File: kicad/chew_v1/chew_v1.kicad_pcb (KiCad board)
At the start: 2 copper layers, 160.3 x 91.9 mm, 44 parts, among them J2 AudioJack4dpb, SW1 SW_Push, SW10 SW_Push, SW11 SW_Push, SW12 SW_Push, SW13 SW_Push, SW14 SW_Push, SW15 SW_Push, SW16 SW_Push, SW17 SW_Push, SW2 SW_Push, SW3 SW_Push, SW4 SW_Push, SW5 SW_Push, SW6 SW_Push, SW7 SW_Push, SW8 SW_Push, SW9 SW_Push

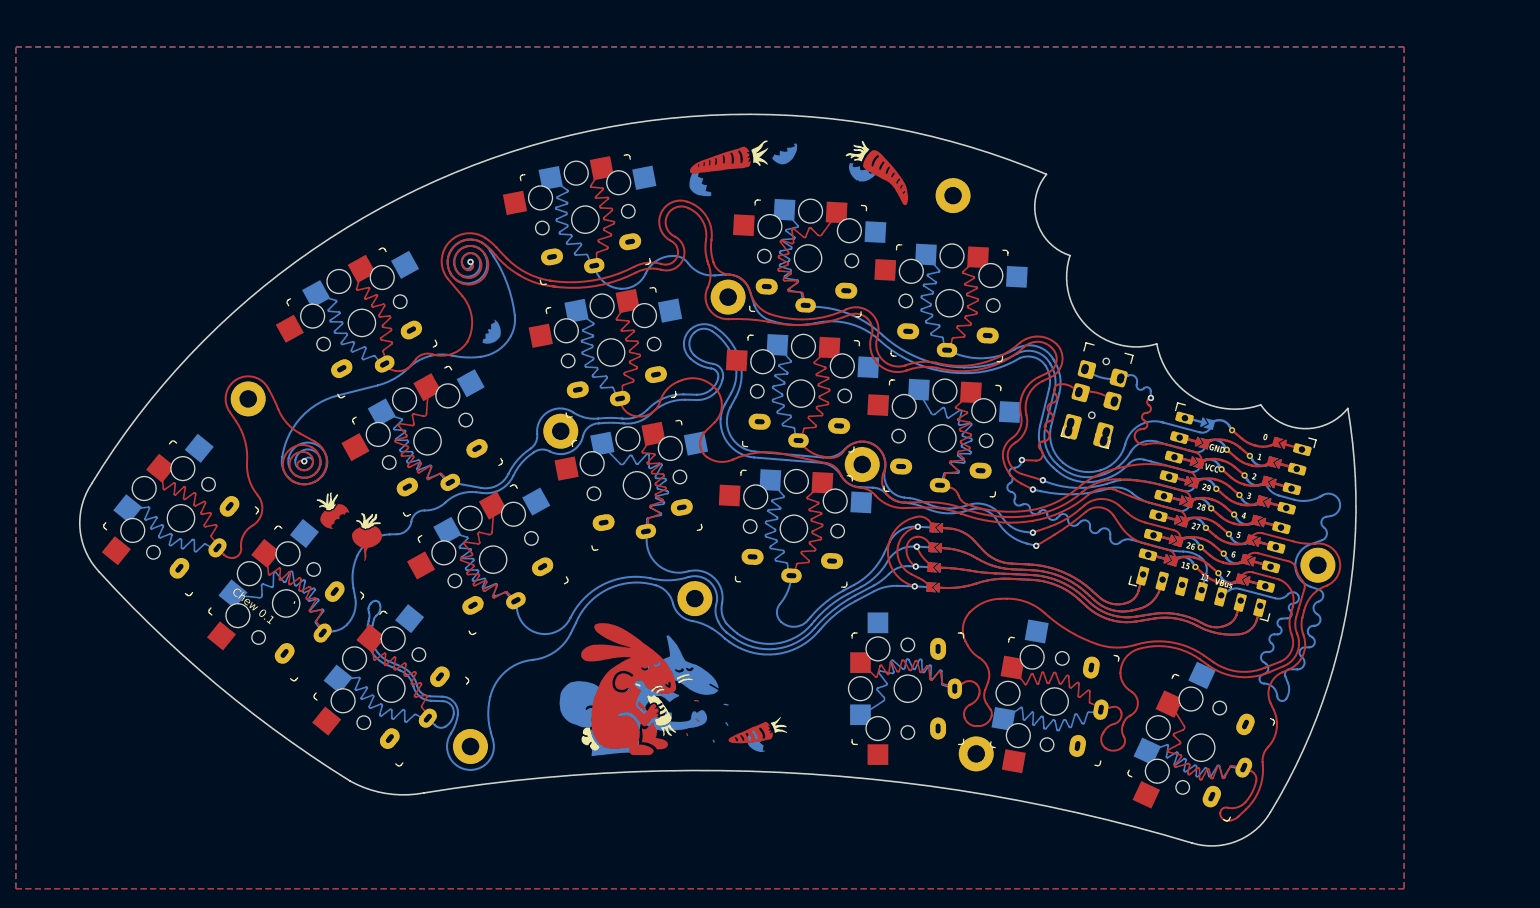
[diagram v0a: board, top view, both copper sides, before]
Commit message: Create libs
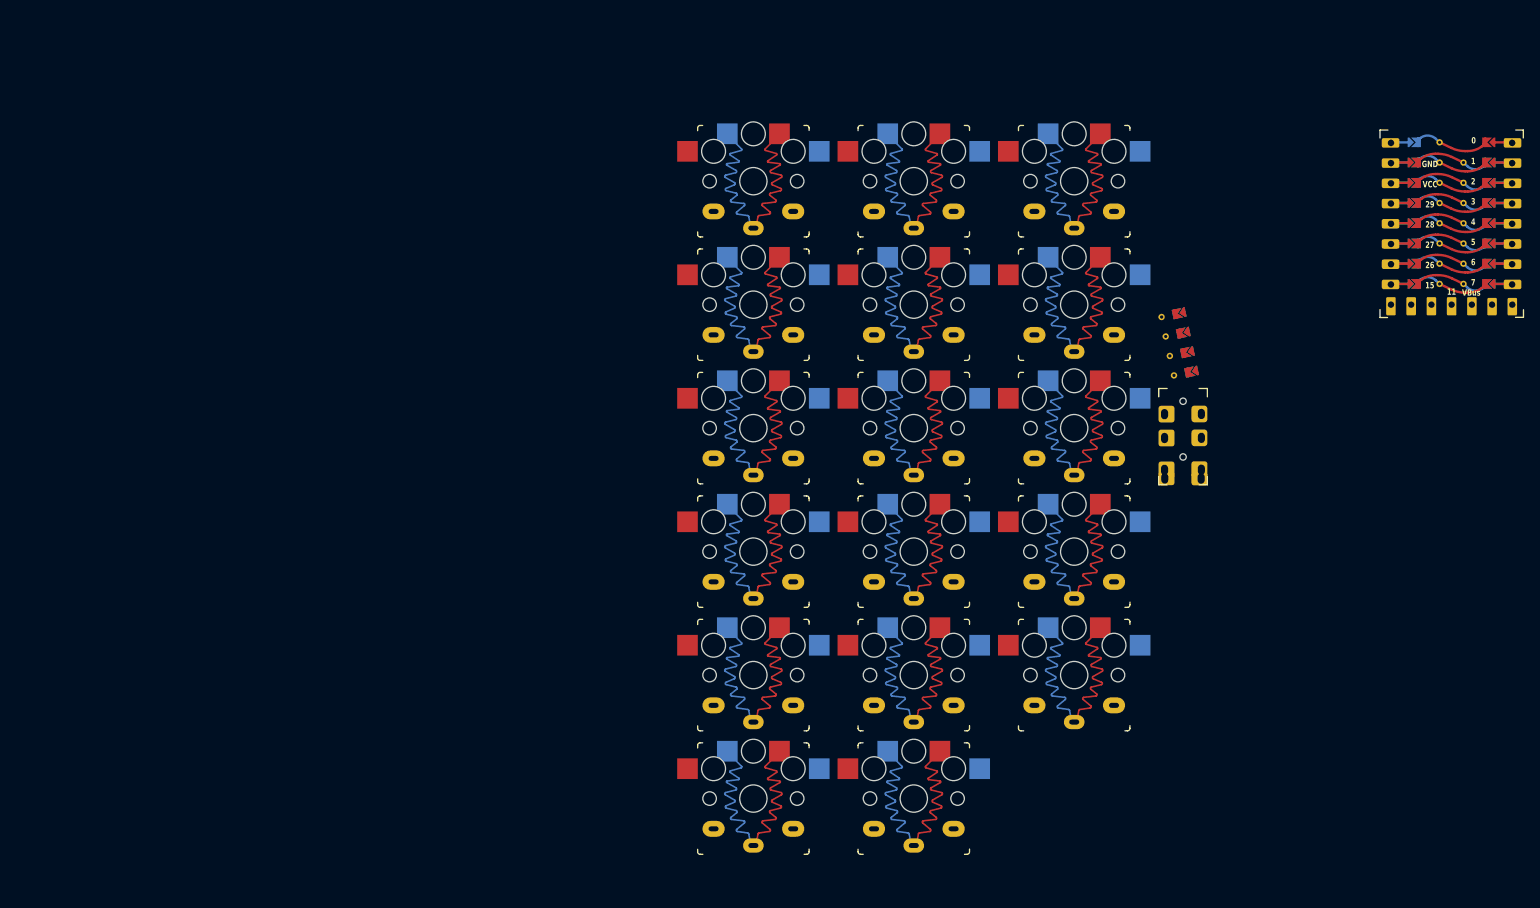
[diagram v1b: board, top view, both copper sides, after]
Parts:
- removed ? (x4): , clipboard:420c2a85-5b5b-48ff-b81a-8100f601aced
- removed ? (x5): , 
- removed G*** (x15): LOGO, LOGO
- removed J2: AudioJack4dpb, Kailh:TRRS-PJ-DPB2
- removed REF**: Tenting Puck, kbd:Tenting_Puck2
- removed RZ1: RP2040-Zero, BumWings_Library:RP2040-Zero
- removed SW1, SW10, SW11, SW12, SW13, SW14, SW15, SW16, SW17, SW2, SW3, SW4, SW5, SW6, SW7, SW8, SW9: SW_Push, * duckyb-collection:SW_PG1350_rev_DPB
- added S1: Keyswitch, chew_is_so:Choc_V1_chew_reversible_1, F.Cu at (113.7, 60.8)
- added S10: Keyswitch, chew_is_so:Choc_V1_chew_reversible_1, F.Cu at (133.9, 107.3)
- added S11: Keyswitch, chew_is_so:Choc_V1_chew_reversible_1, F.Cu at (133.9, 122.8)
- added S12: Keyswitch, chew_is_so:Choc_V1_chew_reversible_1, F.Cu at (133.9, 138.3)
- added S13: Keyswitch, chew_is_so:Choc_V1_chew_reversible_1, F.Cu at (154.0, 60.8)
- added S14: Keyswitch, chew_is_so:Choc_V1_chew_reversible_1, F.Cu at (154.0, 76.3)
- added S15: Keyswitch, chew_is_so:Choc_V1_chew_reversible_1, F.Cu at (154.0, 91.8)
- added S16: Keyswitch, chew_is_so:Choc_V1_chew_reversible_1, F.Cu at (154.0, 107.3)
- added S17: Keyswitch, chew_is_so:Choc_V1_chew_reversible_1, F.Cu at (154.0, 122.8)
- added S2: Keyswitch, chew_is_so:Choc_V1_chew_reversible_1, F.Cu at (113.7, 76.3)
- added S3: Keyswitch, chew_is_so:Choc_V1_chew_reversible_1, F.Cu at (113.7, 91.8)
- added S4: Keyswitch, chew_is_so:Choc_V1_chew_reversible_1, F.Cu at (113.7, 107.3)
- added S5: Keyswitch, chew_is_so:Choc_V1_chew_reversible_1, F.Cu at (113.7, 122.8)
- added S6: Keyswitch, chew_is_so:Choc_V1_chew_reversible_1, F.Cu at (113.7, 138.3)
- added S7: Keyswitch, chew_is_so:Choc_V1_chew_reversible_1, F.Cu at (133.9, 60.8)
- added S8: Keyswitch, chew_is_so:Choc_V1_chew_reversible_1, F.Cu at (133.9, 76.3)
- added S9: Keyswitch, chew_is_so:Choc_V1_chew_reversible_1, F.Cu at (133.9, 91.8)
- added U1: RP2040_Zero, chew_is_so:RP2040_Zero_chew_reversible, F.Cu at (201.4, 66.1)
- added U2: TRRS, chew_is_so:TRRS_chew_reversible, F.Cu at (167.7, 86.8)
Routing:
- net Switch5: track 350.1 -> 0.00 mm, vias 3 -> 0
- net (no net): track 298.2 -> 0.00 mm
- net Switch4: track 169.7 -> 0.00 mm, vias 1 -> 0
- net Switch10: track 157.6 -> 0.00 mm, vias 1 -> 0
- net Switch14: track 144.3 -> 0.00 mm, vias 1 -> 0
- net Switch9: track 133.9 -> 0.00 mm, vias 1 -> 0
- net vcc: track 103.5 -> 0.00 mm, vias 1 -> 0
- net Switch3: track 99.3 -> 0.00 mm
- net Switch8: track 90.2 -> 0.00 mm
- net Switch17: track 86.0 -> 0.00 mm
- net Switch13: track 72.1 -> 0.00 mm, vias 1 -> 0
- net Switch2: track 67.7 -> 0.00 mm
- net Switch16: track 65.5 -> 0.00 mm
- net Switch15: track 61.7 -> 0.00 mm
- net Switch18: track 61.5 -> 0.00 mm, vias 1 -> 0
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- removed copper zone on B.Cu, net gnd
- removed copper zone on F.Cu, net gnd
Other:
- board outline removed
- board text removed: "Chew 0.1"

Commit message: Replace footprints
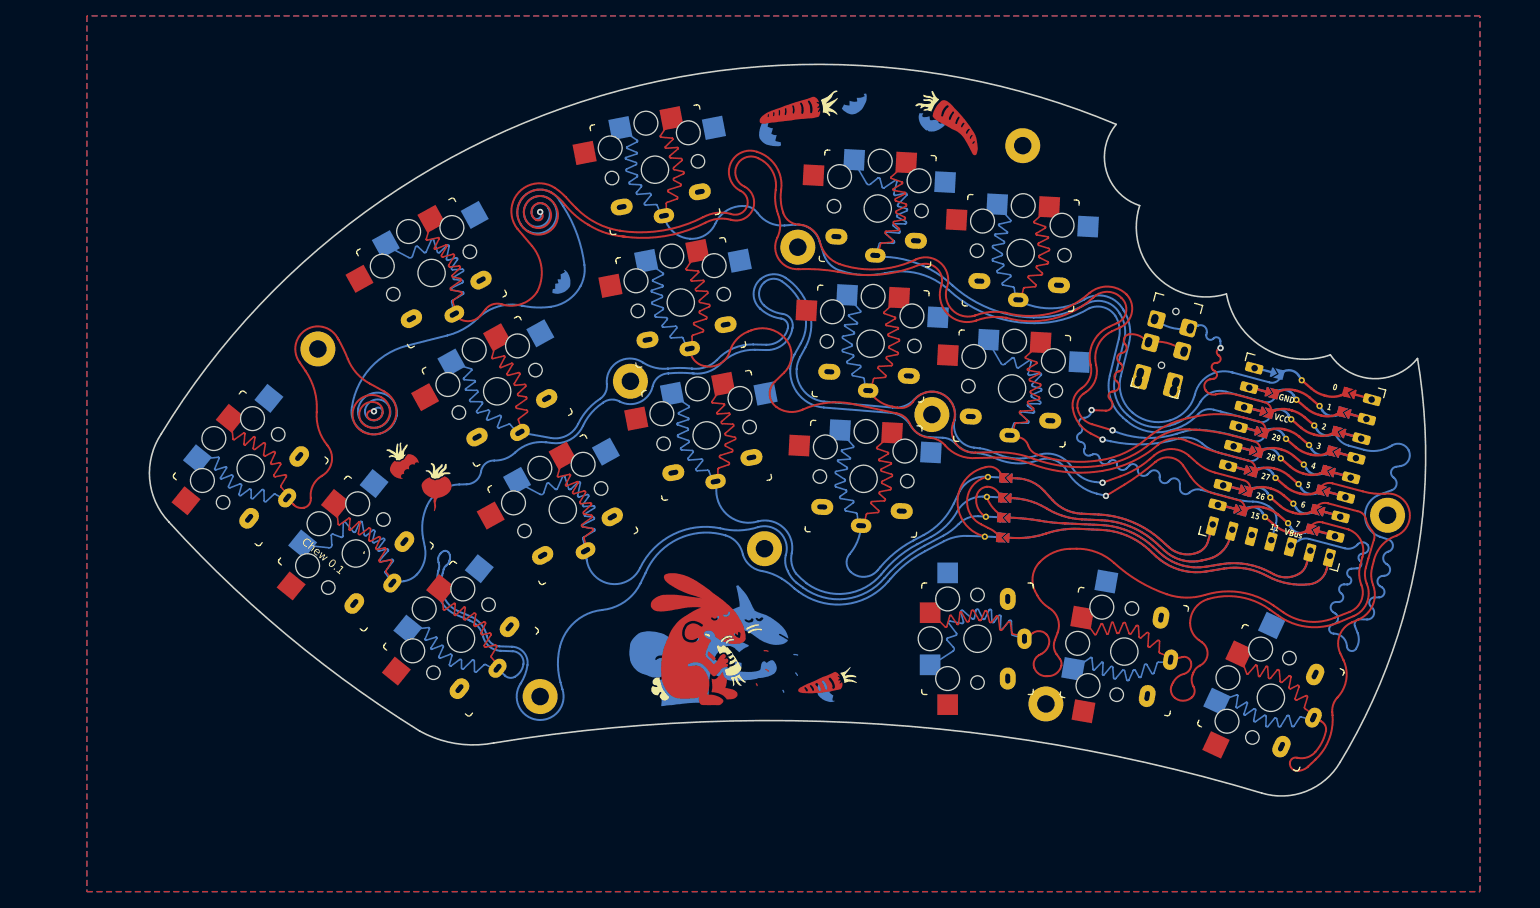
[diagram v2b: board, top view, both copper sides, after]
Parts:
- added ?: , , F.Cu at (86.9, 125.5)
- added ?: , , F.Cu at (193.4, 102.7)
- added ?: , , F.Cu at (147.6, 56.3)
- added ?: , , F.Cu at (150.5, 126.4)
- added ?: , , F.Cu at (59.0, 81.8)
- added G***: LOGO, LOGO, F.Cu at (73.9, 99.1)
- added G***: LOGO, LOGO, B.Cu at (88.9, 72.9)
- added G***: LOGO, LOGO, B.Cu at (76.9, 107.1)
- added G***: LOGO, LOGO, B.Cu at (75.4, 106.0)
- added G***: LOGO, LOGO, B.Cu at (107.7, 117.6)
- added G***: LOGO, LOGO, B.Cu at (123.8, 124.6)
- added G***: LOGO, LOGO, B.Cu at (126.0, 50.2)
- added G***: LOGO, LOGO, F.Cu at (120.0, 50.8)
- added G***: LOGO, LOGO, F.Cu at (69.5, 96.5)
- added G***: LOGO, LOGO, F.Cu at (122.6, 123.7)
- added G***: LOGO, LOGO, F.Cu at (108.2, 117.0)
- added G***: LOGO, LOGO, F.Cu at (137.5, 53.2)
- added G***: LOGO, LOGO, B.Cu at (116.5, 54.6)
- added G***: LOGO, LOGO, B.Cu at (136.4, 52.5)
- added G***: LOGO, LOGO, B.Cu at (76.6, 107.5)
- added REF**: Tenting Puck, kbd:Tenting_Puck2, F.Cu at (117.2, 88.0)
- S10, S13, S15, S2, S4, S6: footprint chew_is_so:Choc_V1_chew_reversible_1 -> chew_is_so:Choc_V1_chew_reversible_2
- moved S14 87.7 mm to (77.0, 118.2), turned to 51 degrees
- moved S13 76.4 mm to (89.8, 102.0), turned to 29 degrees
- moved S10 70.1 mm to (63.8, 107.5), turned to 51 degrees
- moved S5 68.3 mm to (50.6, 96.8), turned to 51 degrees
- moved S6 60.9 mm to (146.2, 86.8), turned to -3 degrees
- moved S4 53.5 mm to (73.3, 72.3), turned to 29 degrees
- moved S9 52.5 mm to (81.5, 87.2), turned to 29 degrees
- moved S12 52.5 mm to (107.9, 92.7), turned to 11 degrees
- moved U1 36.0 mm to (181.4, 96.0), turned to -15 degrees
- moved S1 34.8 mm to (147.3, 69.8), turned to -3 degrees
- moved S3 34.7 mm to (101.4, 59.3), turned to 11 degrees
- moved S8 29.3 mm to (104.6, 76.0), turned to 11 degrees
- moved S15 29.1 mm to (141.9, 118.2), turned to 90 degrees
- moved S11 25.4 mm to (127.6, 98.1), turned to -3 degrees
- moved S17 24.9 mm to (178.7, 125.7), turned to 65 degrees
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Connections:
- S1 pad 1: GND -> S1
- S1 pad 2: S1 -> GND
- S10 pad 1: GND -> S10
- S10 pad 2: S10 -> GND
- S11 pad 1: GND -> S11
- S11 pad 2: S11 -> GND
- S12 pad 1: GND -> S12
- S12 pad 2: S12 -> GND
- S13 pad 1: GND -> S13
- S13 pad 2: S13 -> GND
- S14 pad 1: GND -> S14
- S14 pad 2: S14 -> GND
- S15 pad 1: GND -> S15
- S15 pad 2: S15 -> GND
- S16 pad 1: GND -> S16
- S16 pad 2: S16 -> GND
- S17 pad 1: GND -> S17
- S17 pad 2: S17 -> GND
- S2 pad 1: GND -> S2
- S2 pad 2: S2 -> GND
- S3 pad 1: GND -> S3
- S3 pad 2: S3 -> GND
- S4 pad 1: GND -> S4
- S4 pad 2: S4 -> GND
- S5 pad 1: GND -> S5
- S5 pad 2: S5 -> GND
- S6 pad 1: GND -> S6
- S6 pad 2: S6 -> GND
- S7 pad 1: GND -> S7
- S7 pad 2: S7 -> GND
- S8 pad 1: GND -> S8
- S8 pad 2: S8 -> GND
- S9 pad 1: GND -> S9
- S9 pad 2: S9 -> GND
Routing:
- net S5: track 0.00 -> 350.1 mm, vias 0 -> 1
- net (no net): track 0.00 -> 298.2 mm, vias 0 -> 2
- net S4: track 0.00 -> 169.7 mm, vias 0 -> 1
- net S10: track 0.00 -> 157.6 mm, vias 0 -> 1
- net GND: track 0.00 -> 147.7 mm
- net S14: track 0.00 -> 144.3 mm
- net S9: track 0.00 -> 133.9 mm, vias 0 -> 1
- net VCC: track 0.00 -> 103.5 mm, vias 0 -> 1
- net S3: track 0.00 -> 99.3 mm
- net S8: track 0.00 -> 90.2 mm
- net S13: track 0.00 -> 72.1 mm
- net S2: track 0.00 -> 67.7 mm
- net S16: track 0.00 -> 65.5 mm
- net Comm: track 0.00 -> 61.5 mm, vias 0 -> 1
- net S7: track 0.00 -> 57.7 mm
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- added copper zone on B.Cu, net (none)
- added copper zone on F.Cu, net (none)
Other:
- board outline added: 160.3 x 91.9 mm
- board text added: "Chew 0.1"
